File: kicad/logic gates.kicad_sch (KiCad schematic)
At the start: 33 parts, among them J1 USB_B_Micro, Q1 NPN, Q2 NPN, Q3 NPN, Q4 NPN, Q5 NPN, Q6 NPN, Q7 NPN, SW1 SW_SPST, SW2 SW_SPST, SW3 SW_SPST, SW4 SW_SPST, SW5 SW_SPST, SW6 SW_SPST, SW7 SW_SPST, SW8 SW_DIP_x01

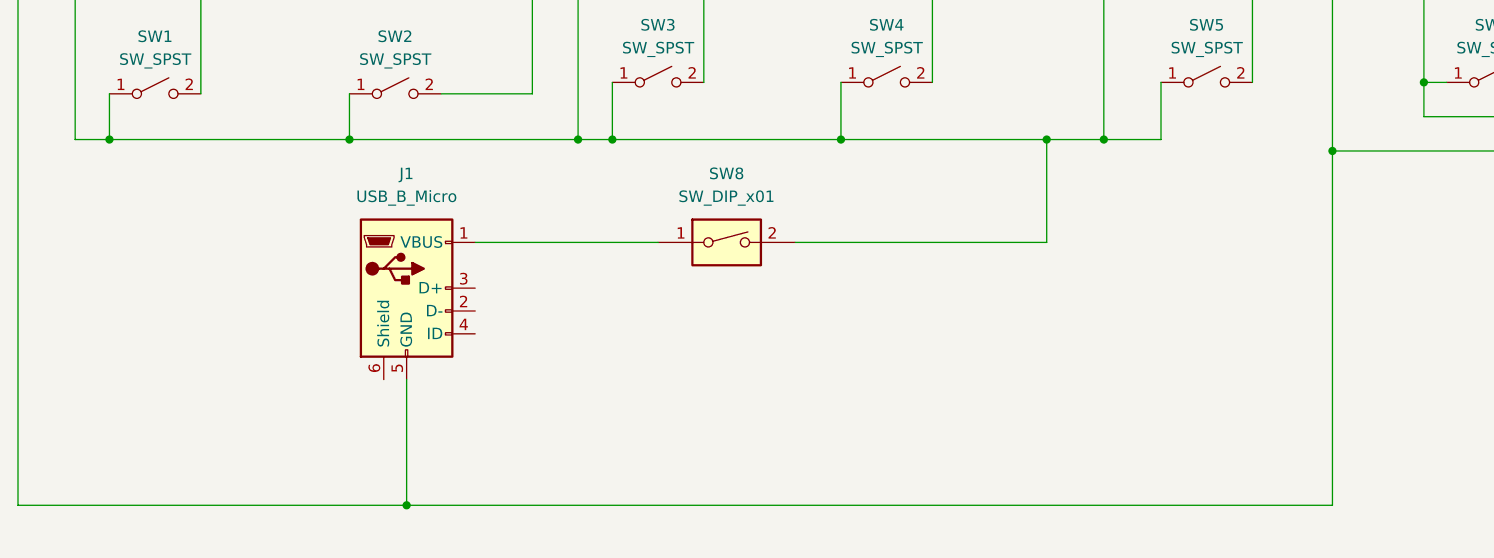
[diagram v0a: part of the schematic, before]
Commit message: fix pcb
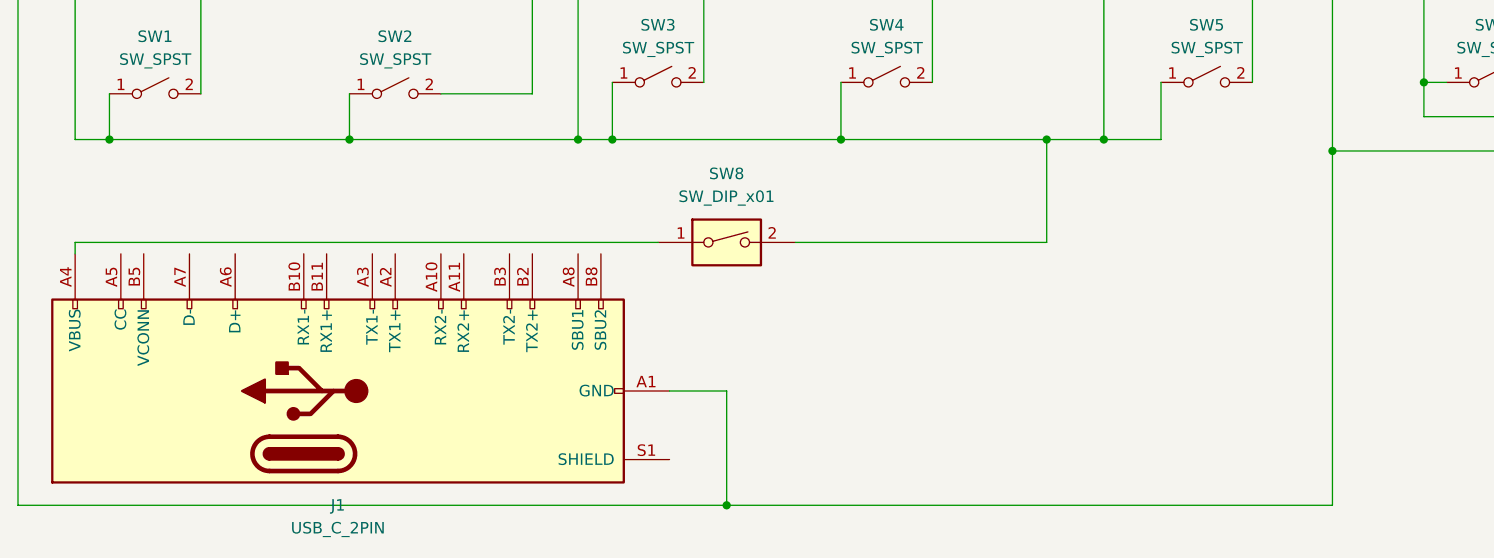
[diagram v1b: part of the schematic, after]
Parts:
- J1: value USB_B_Micro -> USB_C_2PIN; footprint Connector_USB:USB_Mini-B_Tensility_54-00023_Vertical_CircularHoles -> Connector_USB:USB_C_Receptacle_G-Switch_GT-USB-7010ASV; symbol Connector:USB_B_Micro -> Connector:USB_C_Plug
- SW8: footprint Button_Switch_THT:SW_DIP_SPSTx01_Slide_9.78x4.72mm_W7.62mm_P2.54mm -> Button_Switch_THT:SW_CK_JS202011CQN_DPDT_Straight
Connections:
- net at D3.1 (K), Q2.3 (E), Q3.3 (E)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: now also J1.A1 (GND), J1.A12 (GND), J1.B1 (GND), J1.B12 (GND); no longer J1.5 (GND)
- net at SW8.1: now also J1.A4 (VBUS), J1.A9 (VBUS), J1.B4 (VBUS), J1.B9 (VBUS); no longer J1.1 (VBUS)
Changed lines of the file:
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@@
+	)
+	(junction
+		(at 100.33 187.96)
+		(diameter 0)
+		(color 0 0 0 0)
 	)
 	(junction
@@
 	)
 	(junction
-		(at 64.77 187.96)
-		(diameter 0)
-		(color 0 0 0 0)
-	)
-	(junction
 		(at 187.96 21.59)
 		(diameter 0)
@@
 	(wire
 		(pts
+			(xy 93.98 175.26) (xy 100.33 175.26)
+		)
+		(stroke
+			(width 0)
+			(type default)
+		)
+	)
+	(wire
+		(pts
 			(xy 154.94 92.71) (xy 154.94 119.38)
 		)
@@
 	(wire
 		(pts
-			(xy 167.64 187.96) (xy 64.77 187.96)
+			(xy 21.59 187.96) (xy 100.33 187.96)
 		)
 		(stroke
@@
 	(wire
 		(pts
-			(xy 64.77 187.96) (xy 21.59 187.96)
-		)
-		(stroke
-			(width 0)
-			(type default)
-		)
-	)
-	(wire
-		(pts
 			(xy 83.82 147.32) (xy 87.63 147.32)
 		)
@@
 	(wire
 		(pts
-			(xy 64.77 173.99) (xy 64.77 187.96)
-		)
-		(stroke
-			(width 0)
-			(type default)
-		)
-	)
-	(wire
-		(pts
 			(xy 227.33 54.61) (xy 227.33 69.85)
 		)
@@
 	(wire
 		(pts
+			(xy 92.71 158.75) (xy 27.94 158.75)
+		)
+		(stroke
+			(width 0)
+			(type default)
+		)
+	)
+	(wire
+		(pts
 			(xy 251.46 66.04) (xy 251.46 110.49)
 		)
@@
 	(wire
 		(pts
+			(xy 27.94 158.75) (xy 27.94 160.02)
+		)
+		(stroke
+			(width 0)
+			(type default)
+		)
+	)
+	(wire
+		(pts
 			(xy 227.33 21.59) (xy 227.33 38.1)
 		)
@@
 	(wire
 		(pts
+			(xy 100.33 175.26) (xy 100.33 187.96)
+		)
+		(stroke
+			(width 0)
+			(type default)
+		)
+	)
+	(wire
+		(pts
 			(xy 78.74 127) (xy 78.74 142.24)
 		)
@@
 	(wire
 		(pts
-			(xy 72.39 158.75) (xy 92.71 158.75)
-		)
-		(stroke
-			(width 0)
-			(type default)
-		)
-	)
-	(wire
-		(pts
 			(xy 160.02 21.59) (xy 187.96 21.59)
 		)
@@
 		(pts
 			(xy 142.24 21.59) (xy 142.24 147.32)
+		)
+		(stroke
+			(width 0)
+			(type default)
+		)
+	)
+	(wire
+		(pts
+			(xy 100.33 187.96) (xy 167.64 187.96)
 		)
 		(stroke
@@
 			)
 		)
-		(property "Footprint" "Button_Switch_THT:SW_DIP_SPSTx01_Slide_9.78x4.72mm_W7.62mm_P2.54mm"
+		(property "Footprint" "Button_Switch_THT:SW_CK_JS202011CQN_DPDT_Straight"
 			(at 100.33 158.75 0)
 			(effects
@@
 	)
 	(symbol
-		(lib_id "Connector:USB_B_Micro")
-		(at 64.77 163.83 0)
+		(lib_id "Connector:USB_C_Plug")
+		(at 53.34 175.26 90)
 		(unit 1)
 		(exclude_from_sim no)
@@
 		(fields_autoplaced yes)
 		(property "Reference" "J1"
-			(at 64.77 151.13 0)
-			(effects
-				(font
-					(size 1.27 1.27)
-				)
-			)
-		)
-		(property "Value" "USB_B_Micro"
-			(at 64.77 153.67 0)
-			(effects
-				(font
-					(size 1.27 1.27)
-				)
-			)
-		)
-		(property "Footprint" "Connector_USB:USB_Mini-B_Tensility_54-00023_Vertical_CircularHoles"
-			(at 68.58 165.1 0)
-			(effects
-				(font
-					(size 1.27 1.27)
-				)
-				(hide yes)
-			)
-		)
-		(property "Datasheet" "~"
-			(at 68.58 165.1 0)
-			(effects
-				(font
-					(size 1.27 1.27)
-				)
-				(hide yes)
-			)
-		)
-		(property "Description" "USB Micro Type B connector"
-			(at 64.77 163.83 0)
-			(effects
-				(font
-					(size 1.27 1.27)
-				)
-				(hide yes)
-			)
-		)
-		(pin "5"
-		)
-		(pin "1"
-		)
-		(pin "4"
-		)
-		(pin "3"
-		)
-		(pin "6"
-		)
-		(pin "2"
+			(at 57.15 187.96 90)
+			(effects
+				(font
+					(size 1.27 1.27)
+				)
+			)
+		)
+		(property "Value" "USB_C_2PIN"
+			(at 57.15 190.5 90)
+			(effects
+				(font
+					(size 1.27 1.27)
+				)
+			)
+		)
+		(property "Footprint" "Connector_USB:USB_C_Receptacle_G-Switch_GT-USB-7010ASV"
+			(at 53.34 171.45 0)
+			(effects
+				(font
+					(size 1.27 1.27)
+				)
+				(hide yes)
+			)
+		)
+		(property "Datasheet" "https://www.usb.org/sites/default/files/documents/usb_type-c.zip"
+			(at 53.34 171.45 0)
+			(effects
+				(font
+					(size 1.27 1.27)
+				)
+				(hide yes)
+			)
+		)
+		(property "Description" "USB Type-C Plug connector"
+			(at 53.34 175.26 0)
+			(effects
+				(font
+					(size 1.27 1.27)
+				)
+				(hide yes)
+			)
+		)
+		(pin "A4"
+		)
+		(pin "A3"
+		)
+		(pin "A2"
+		)
+		(pin "A10"
+		)
+		(pin "B2"
+		)
+		(pin "B5"
+		)
+		(pin "A12"
+		)
+		(pin "A11"
+		)
+		(pin "B12"
+		)
+		(pin "A9"
+		)
+		(pin "B1"
+		)
+		(pin "B10"
+		)
+		(pin "B11"
+		)
+		(pin "B4"
+		)
+		(pin "A7"
+		)
+		(pin "A5"
+		)
+		(pin "A6"
+		)
+		(pin "A8"
+		)
+		(pin "B8"
+		)
+		(pin "A1"
+		)
+		(pin "B9"
+		)
+		(pin "S1"
+		)
+		(pin "B3"
 		)
 		(instances
